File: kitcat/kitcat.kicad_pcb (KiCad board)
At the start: 2 copper layers, 46.5 x 59 mm, 29 parts, among them IC1 LA4182, J1 Conn_01x02, J2 Conn_01x02, J3 Conn_01x02, J4 Conn_01x02, J5 Conn_01x02

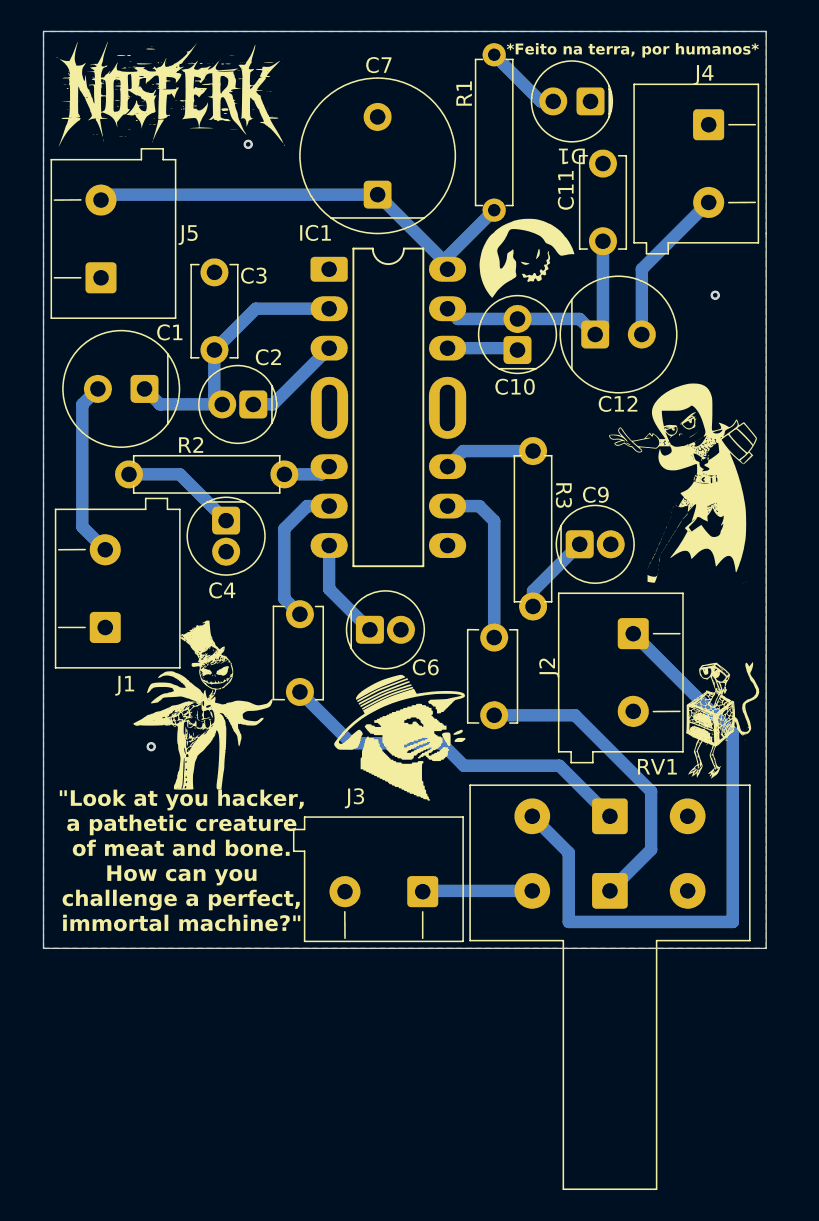
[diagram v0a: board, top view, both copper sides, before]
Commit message: fyj
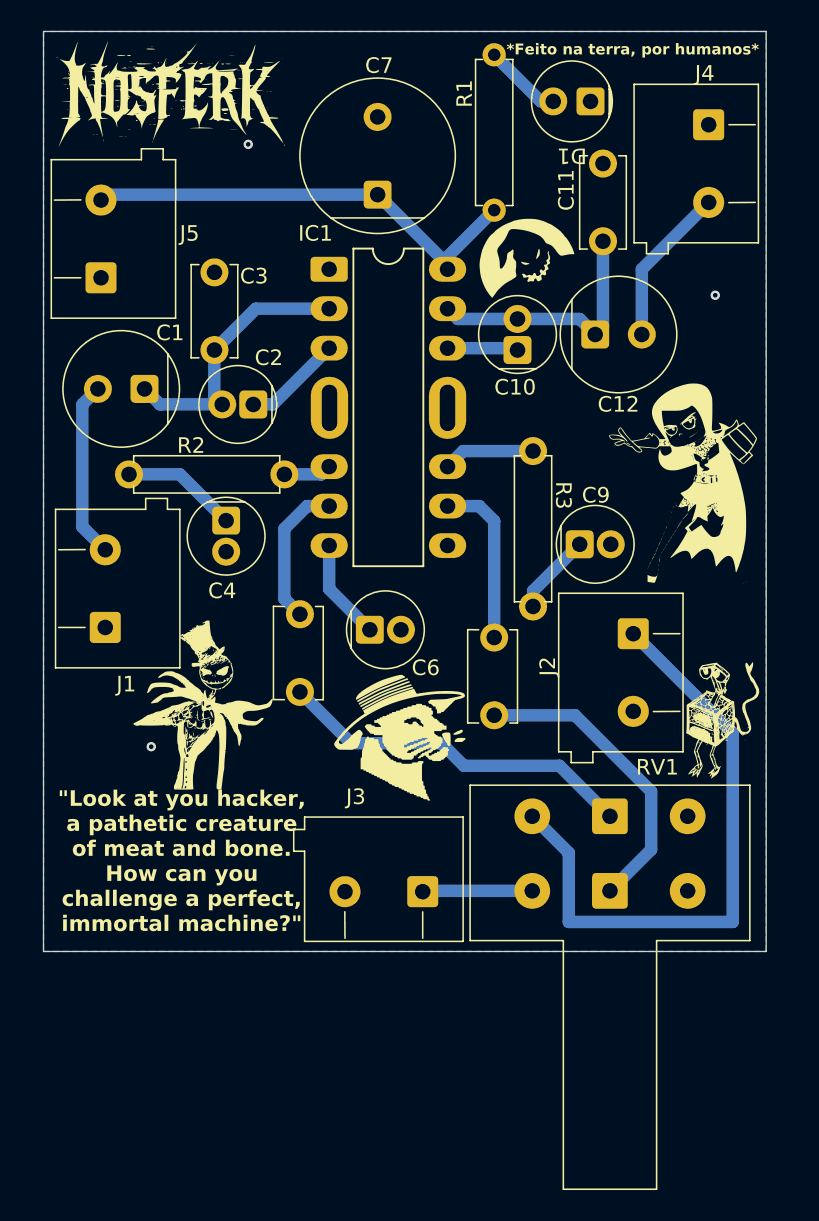
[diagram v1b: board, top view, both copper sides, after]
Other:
- board size 46.5 x 59 mm -> 46.5 x 59.2 mm
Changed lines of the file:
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@@
 	)
 	(gr_line
-		(start 197 72)
-		(end 197 118)
+		(start 197 59)
+		(end 197 118.2)
 		(stroke
 			(width 0.05)
@@
 	)
 	(gr_line
-		(start 150.5 118)
+		(start 150.5 118.2)
 		(end 150.5 59)
 		(stroke
@@
 	)
 	(gr_line
-		(start 197 59)
-		(end 197 72)
-		(stroke
-			(width 0.05)
-			(type default)
-		)
-		(layer "Edge.Cuts")
-	)
-	(gr_line
-		(start 197 118)
-		(end 150.5 118)
+		(start 197 118.2)
+		(end 150.5 118.2)
 		(stroke
 			(width 0.05)
@@
 		(polygon
 			(pts
-				(xy 197 118) (xy 197 59) (xy 150.5 59) (xy 150.5 118)
+				(xy 197 118.2) (xy 197 59) (xy 150.5 59) (xy 150.5 118.2)
 			)
 		)
